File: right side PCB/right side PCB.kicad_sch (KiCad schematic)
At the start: 5 parts, among them J1 Conn_02x02_Counter_Clockwise, U11 LD1117S50TR_SOT223

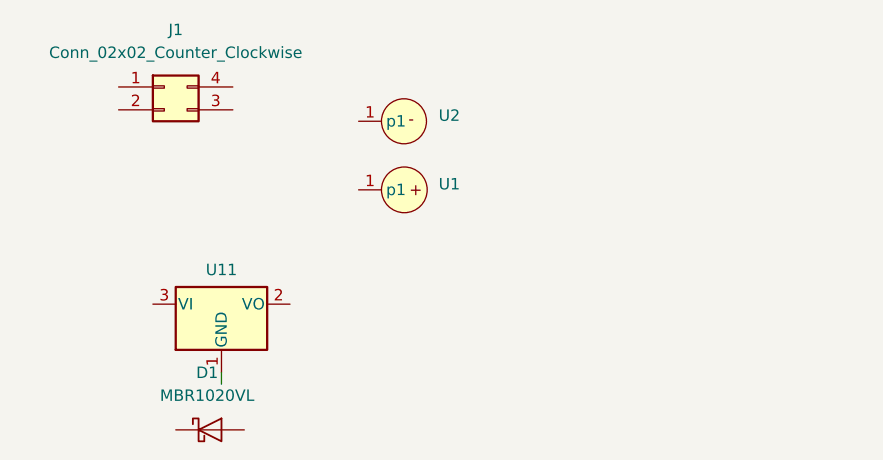
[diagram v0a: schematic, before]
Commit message: boxpcb
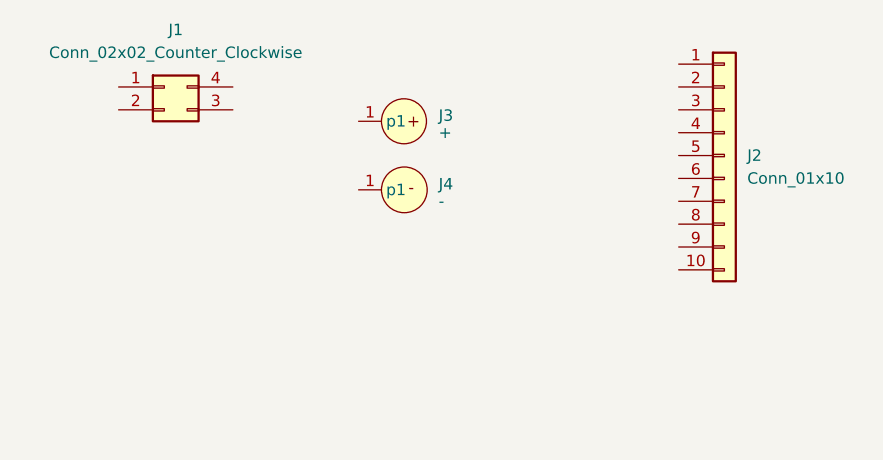
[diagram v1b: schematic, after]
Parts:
- removed D1: MBR1020VL, Diode_SMD:D_SOD-123F, symbol Diode:MBR1020VL
- removed U11: LD1117S50TR_SOT223, power_bl:SOT-223-3_TabPin2, symbol power_bl:LD1117S50TR_SOT223
- added J2: Conn_01x10, Connector_PinHeader_2.00mm:PinHeader_1x10_P2.00mm_Vertical, symbol Connector_Generic:Conn_01x10
- J3: renamed from U2; value ~ -> +
- J4: renamed from U1; value ~ -> -
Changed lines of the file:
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@@
 	(generator_version "8.0")
 	(paper "A4")
-	(wire
-		(pts
-			(xy 119.38 107.95) (xy 119.38 106.68)
-		)
-		(stroke
-			(width 0)
-			(type default)
-		)
-	)
-	(symbol
-		(lib_id "Diode:MBR1020VL")
-		(at 118.11 113.03 0)
-		(unit 1)
-		(exclude_from_sim no)
-		(in_bom yes)
-		(on_board yes)
-		(dnp no)
-		(fields_autoplaced yes)
-		(property "Reference" "D1"
-			(at 117.7925 106.68 0)
-			(effects
-				(font
-					(size 1.27 1.27)
-				)
-			)
-		)
-		(property "Value" "MBR1020VL"
-			(at 117.7925 109.22 0)
-			(effects
-				(font
-					(size 1.27 1.27)
-				)
-			)
-		)
-		(property "Footprint" "Diode_SMD:D_SOD-123F"
-			(at 118.11 117.475 0)
-			(effects
-				(font
-					(size 1.27 1.27)
-				)
-				(hide yes)
-			)
-		)
-		(property "Datasheet" "https://www.onsemi.com/pub/Collateral/MBR1020VL-D.PDF"
-			(at 118.11 113.03 0)
-			(effects
-				(font
-					(size 1.27 1.27)
-				)
-				(hide yes)
-			)
-		)
-		(property "Description" ""
-			(at 118.11 113.03 0)
-			(effects
-				(font
-					(size 1.27 1.27)
-				)
-				(hide yes)
-			)
-		)
-		(pin "1"
-		)
-		(pin "2"
-		)
-		(instances
-			(project ""
-				(path "/3371d9f1-4ea1-4b23-b105-1bd8a9fee2a2"
-					(reference "D1")
-					(unit 1)
-				)
-			)
-		)
-	)
-	(symbol
-		(lib_id "power_bl:LD1117S50TR_SOT223")
-		(at 119.38 99.06 0)
-		(unit 1)
-		(exclude_from_sim no)
-		(in_bom yes)
-		(on_board yes)
-		(dnp no)
-		(fields_autoplaced yes)
-		(property "Reference" "U11"
-			(at 119.38 95.25 0)
-			(effects
-				(font
-					(size 1.27 1.27)
-				)
-			)
-		)
-		(property "Value" "LD1117S50TR_SOT223"
-			(at 119.38 93.98 0)
-			(effects
-				(font
-					(size 1.27 1.27)
-				)
-				(hide yes)
-			)
-		)
-		(property "Footprint" "power_bl:SOT-223-3_TabPin2"
-			(at 119.38 93.98 0)
-			(effects
-				(font
-					(size 1.27 1.27)
-				)
-				(hide yes)
-			)
-		)
-		(property "Datasheet" "http://www.st.com/st-web-ui/static/active/en/resource/technical/document/datasheet/CD00000544.pdf"
-			(at 121.92 105.41 0)
-			(effects
-				(font
-					(size 1.27 1.27)
-				)
-				(hide yes)
-			)
-		)
-		(property "Description" ""
-			(at 119.38 99.06 0)
-			(effects
-				(font
-					(size 1.27 1.27)
-				)
-				(hide yes)
-			)
-		)
-		(pin "3"
-		)
-		(pin "2"
-		)
-		(pin "1"
-		)
-		(instances
-			(project ""
-				(path "/3371d9f1-4ea1-4b23-b105-1bd8a9fee2a2"
-					(reference "U11")
-					(unit 1)
-				)
-			)
-		)
-	)
 	(symbol
 		(lib_id "supply_btr:conn_min")
@@
 		(dnp no)
 		(fields_autoplaced yes)
-		(property "Reference" "U2"
+		(property "Reference" "J3"
 			(at 143.51 78.1049 0)
 			(effects
@@
 			)
 		)
-		(property "Value" "~"
+		(property "Value" "+"
 			(at 143.51 80.01 0)
 			(effects
@@
 			(project ""
 				(path "/3371d9f1-4ea1-4b23-b105-1bd8a9fee2a2"
-					(reference "U2")
+					(reference "J3")
 					(unit 1)
 				)
@@
 		(dnp no)
 		(fields_autoplaced yes)
-		(property "Reference" "U1"
+		(property "Reference" "J4"
 			(at 143.51 85.7249 0)
 			(effects
@@
 			)
 		)
-		(property "Value" "~"
+		(property "Value" "-"
 			(at 143.51 87.63 0)
 			(effects
@@
 			(project ""
 				(path "/3371d9f1-4ea1-4b23-b105-1bd8a9fee2a2"
-					(reference "U1")
-					(unit 1)
-				)
+					(reference "J4")
+					(unit 1)
+				)
+			)
+		)
+	)
+	(symbol
+		(lib_id "Connector_Generic:Conn_01x10")
+		(at 175.26 82.55 0)
+		(unit 1)
+		(exclude_from_sim no)
+		(in_bom yes)
+		(on_board yes)
+		(dnp no)
+		(fields_autoplaced yes)
+		(property "Reference" "J2"
+			(at 177.8 82.5499 0)
+			(effects
+				(font
+					(size 1.27 1.27)
+				)
+				(justify left)
+			)
+		)
+		(property "Value" "Conn_01x10"
+			(at 177.8 85.0899 0)
+			(effects
+				(font
+					(size 1.27 1.27)
+				)
+				(justify left)
+			)
+		)
+		(property "Footprint" "Connector_PinHeader_2.00mm:PinHeader_1x10_P2.00mm_Vertical"
+			(at 175.26 82.55 0)
+			(effects
+				(font
+					(size 1.27 1.27)
+				)
+				(hide yes)
+			)
+		)
+		(property "Datasheet" "~"
+			(at 175.26 82.55 0)
+			(effects
+				(font
+					(size 1.27 1.27)
+				)
+				(hide yes)
+			)
+		)
+		(property "Description" "Generic connector, single row, 01x10, script generated (kicad-library-utils/schlib/autogen/connector/)"
+			(at 175.26 82.55 0)
+			(effects
+				(font
+					(size 1.27 1.27)
+				)
+				(hide yes)
+			)
+		)
+		(pin "6"
+		)
+		(pin "8"
+		)
+		(pin "5"
+		)
+		(pin "1"
+		)
+		(pin "9"
+		)
+		(pin "3"
+		)
+		(pin "10"
+		)
+		(pin "4"
+		)
+		(pin "2"
+		)
+		(pin "7"
+		)
+		(instances
+			(project ""
+				(path "/3371d9f1-4ea1-4b23-b105-1bd8a9fee2a2"
+					(reference "J2")
+					(unit 1)
+				)
